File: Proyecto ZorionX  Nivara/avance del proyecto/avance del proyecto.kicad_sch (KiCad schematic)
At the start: 7 parts, among them J1 24VDC, J2 Screw_Terminal_01x03, J3 Screw_Terminal_01x04, J4 Screw_Terminal_01x06, J5 Screw_Terminal_01x02, J6 Screw_Terminal_01x02, J7 Screw_Terminal_01x02

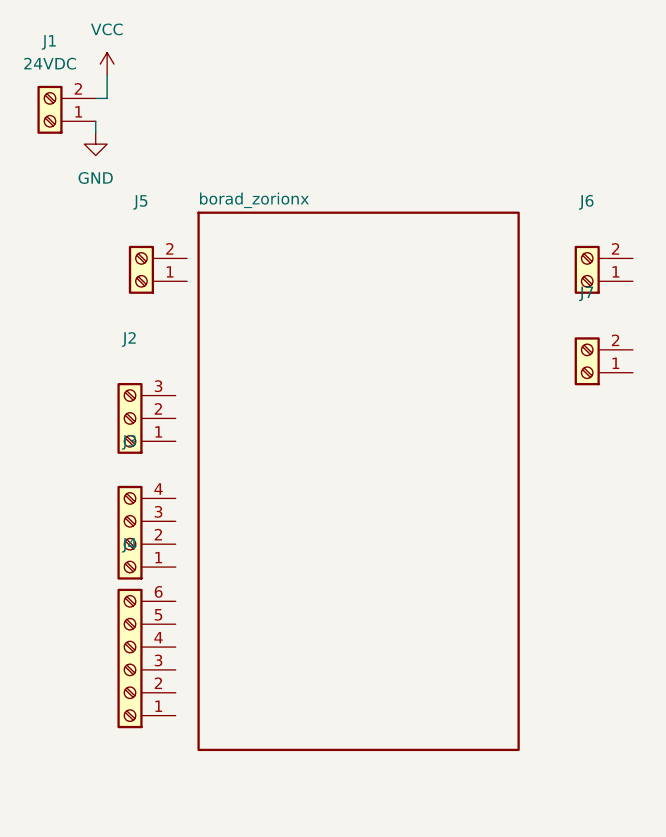
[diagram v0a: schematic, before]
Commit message: Add files via upload
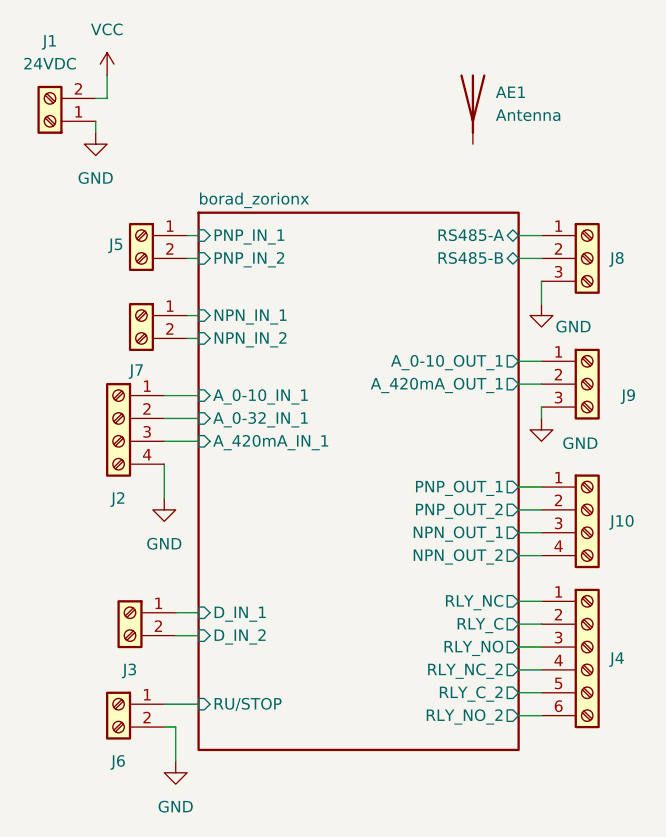
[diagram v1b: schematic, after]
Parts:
- removed J2: Screw_Terminal_01x03, symbol Connector:Screw_Terminal_01x03
- removed J3: Screw_Terminal_01x04, symbol Connector:Screw_Terminal_01x04
- added AE1: Antenna, symbol Device:Antenna
- added J10, J2: Screw_Terminal_01x04, TerminalBlock:TerminalBlock_bornier-4_P5.08mm, symbol Connector:Screw_Terminal_01x04
- added J3: Screw_Terminal_01x02, TerminalBlock:TerminalBlock_bornier-2_P5.08mm, symbol Connector:Screw_Terminal_01x02
- added J8, J9: Screw_Terminal_01x03, TerminalBlock:TerminalBlock_bornier-3_P5.08mm, symbol Connector:Screw_Terminal_01x03
- J1, J5, J6, J7: footprint (none) -> TerminalBlock:TerminalBlock_bornier-2_P5.08mm
- J4: footprint (none) -> TerminalBlock:TerminalBlock_bornier-6_P5.08mm
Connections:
- net GND: now also J6.2 (Pin_2), J2.4 (Pin_4), J8.3 (Pin_3), J9.3 (Pin_3)
- net borad_zorionx/RLY_NC: now reaches J4.1 (Pin_1)
- net borad_zorionx/RLY_C: now reaches J4.2 (Pin_2)
- net borad_zorionx/RLY_NO: now reaches J4.3 (Pin_3)
- net borad_zorionx/RLY_NC_2: now reaches J4.4 (Pin_4)
- net borad_zorionx/RLY_C_2: now reaches J4.5 (Pin_5)
- net borad_zorionx/RLY_NO_2: now reaches J4.6 (Pin_6)
- net borad_zorionx/NPN_IN_1: now reaches J7.1 (Pin_1)
- net borad_zorionx/NPN_IN_2: now reaches J7.2 (Pin_2)
- net borad_zorionx/PNP_IN_1: now reaches J5.1 (Pin_1)
- net borad_zorionx/PNP_IN_2: now reaches J5.2 (Pin_2)
- net borad_zorionx/RU/STOP: now reaches J6.1 (Pin_1)
- new net borad_zorionx/A_0-10_IN_1: J2.1 (Pin_1)
- new net borad_zorionx/A_0-10_OUT_1: J9.1 (Pin_1)
- new net borad_zorionx/A_0-32_IN_1: J2.2 (Pin_2)
- new net borad_zorionx/A_420mA_IN_1: J2.3 (Pin_3)
- new net borad_zorionx/A_420mA_OUT_1: J9.2 (Pin_2)
- new net borad_zorionx/D_IN_1: J3.1 (Pin_1)
- new net borad_zorionx/D_IN_2: J3.2 (Pin_2)
- new net borad_zorionx/NPN_OUT_1: J10.3 (Pin_3)
- new net borad_zorionx/NPN_OUT_2: J10.4 (Pin_4)
- new net borad_zorionx/PNP_OUT_1: J10.1 (Pin_1)
- new net borad_zorionx/PNP_OUT_2: J10.2 (Pin_2)
- new net borad_zorionx/RS485-A: J8.1 (Pin_1)
- new net borad_zorionx/RS485-B: J8.2 (Pin_2)
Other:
- sheet borad_zorionx ports: added A_0-10_IN_1, A_0-10_OUT_1, A_0-32_IN_1, A_420mA_IN_1, A_420mA_OUT_1, D_IN_1, D_IN_2, NPN_IN_1, NPN_IN_2, NPN_OUT_1, NPN_OUT_2, PNP_IN_1, PNP_IN_2, PNP_OUT_1, PNP_OUT_2, RLY_C, RLY_C_2, RLY_NC, RLY_NC_2, RLY_NO, RLY_NO_2, RS485-A, RS485-B, RU/STOP; removed none
- moved on the sheet: J4, J5, J6, J7
